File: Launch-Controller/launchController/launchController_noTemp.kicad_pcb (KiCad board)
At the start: 4 copper layers, 226 x 138.5 mm, 103 parts, among them J1 Conn_01x05_Pin, J10 Conn_01x05_Pin, J11 Raspberry_Pi_5, J13 26 pin Dsub, J14 DB25_Plug, J16 DB25_Plug, J17 DB25_Plug, J2 Conn_01x05_Pin, J3 Conn_01x05_Pin, J4 Conn_01x05_Pin, J5 Conn_01x05_Pin, J6 Conn_01x05_Pin, J7 Conn_01x05_Pin, J8 Conn_01x05_Pin, J9 Conn_01x05_Pin, Q1 NFET, Q10 NFET, Q2 NFET, Q3 NFET, Q4 NFET, Q5 NFET, Q6 NFET, Q7 NFET, Q8 NFET, Q9 NFET, U1 ADS1015IDGS, U2 ADS1015IDGS

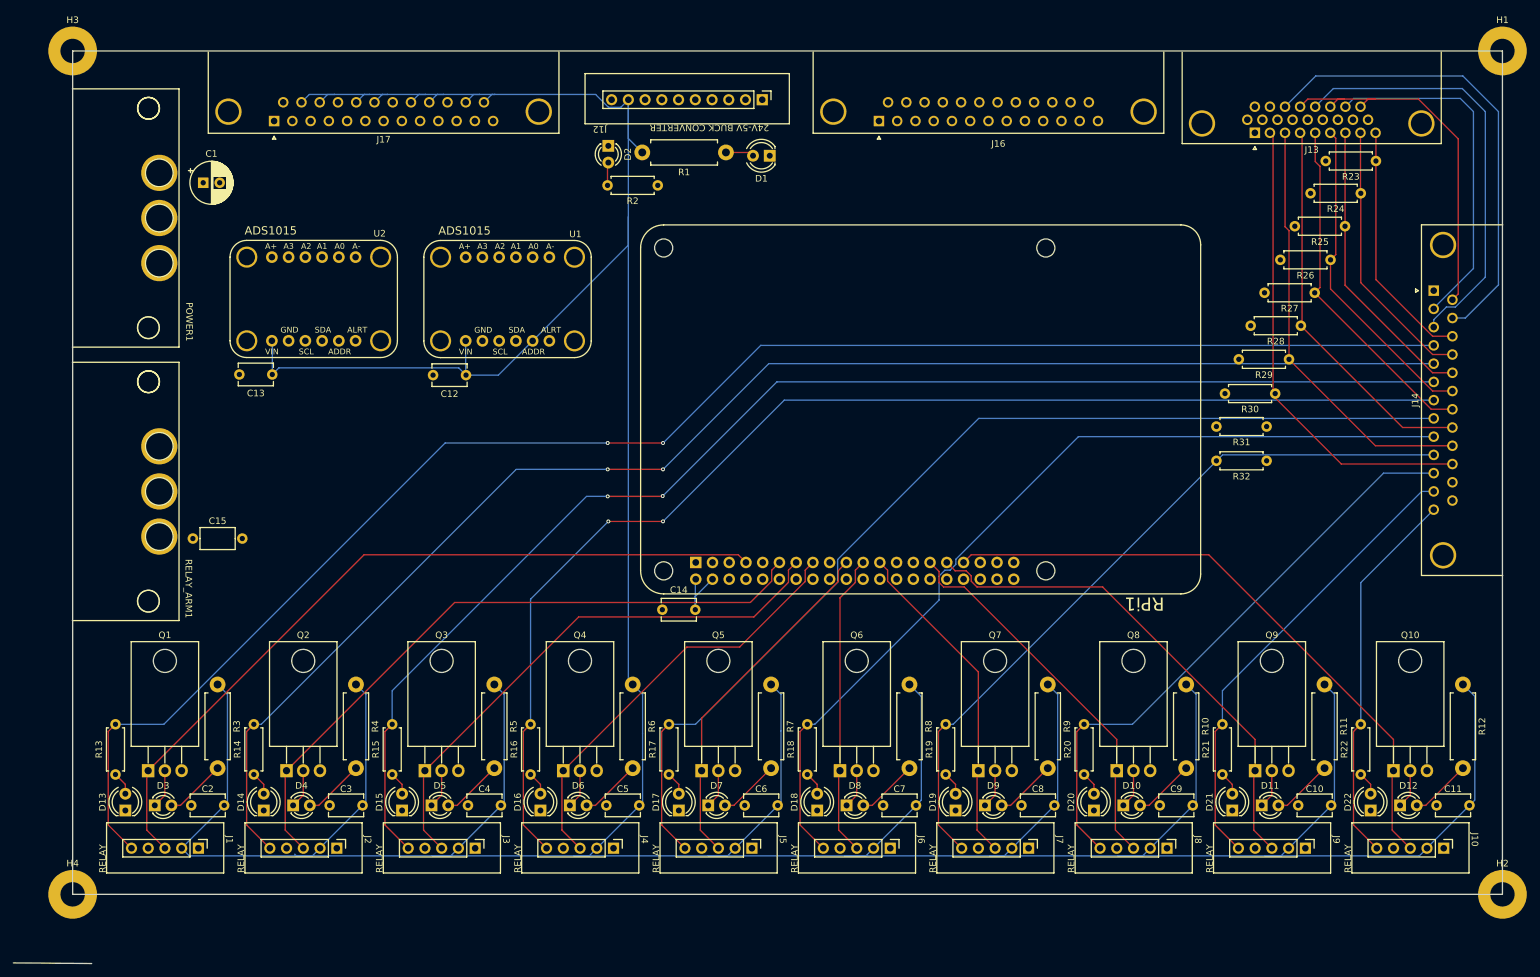
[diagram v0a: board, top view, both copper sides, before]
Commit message: dimensions
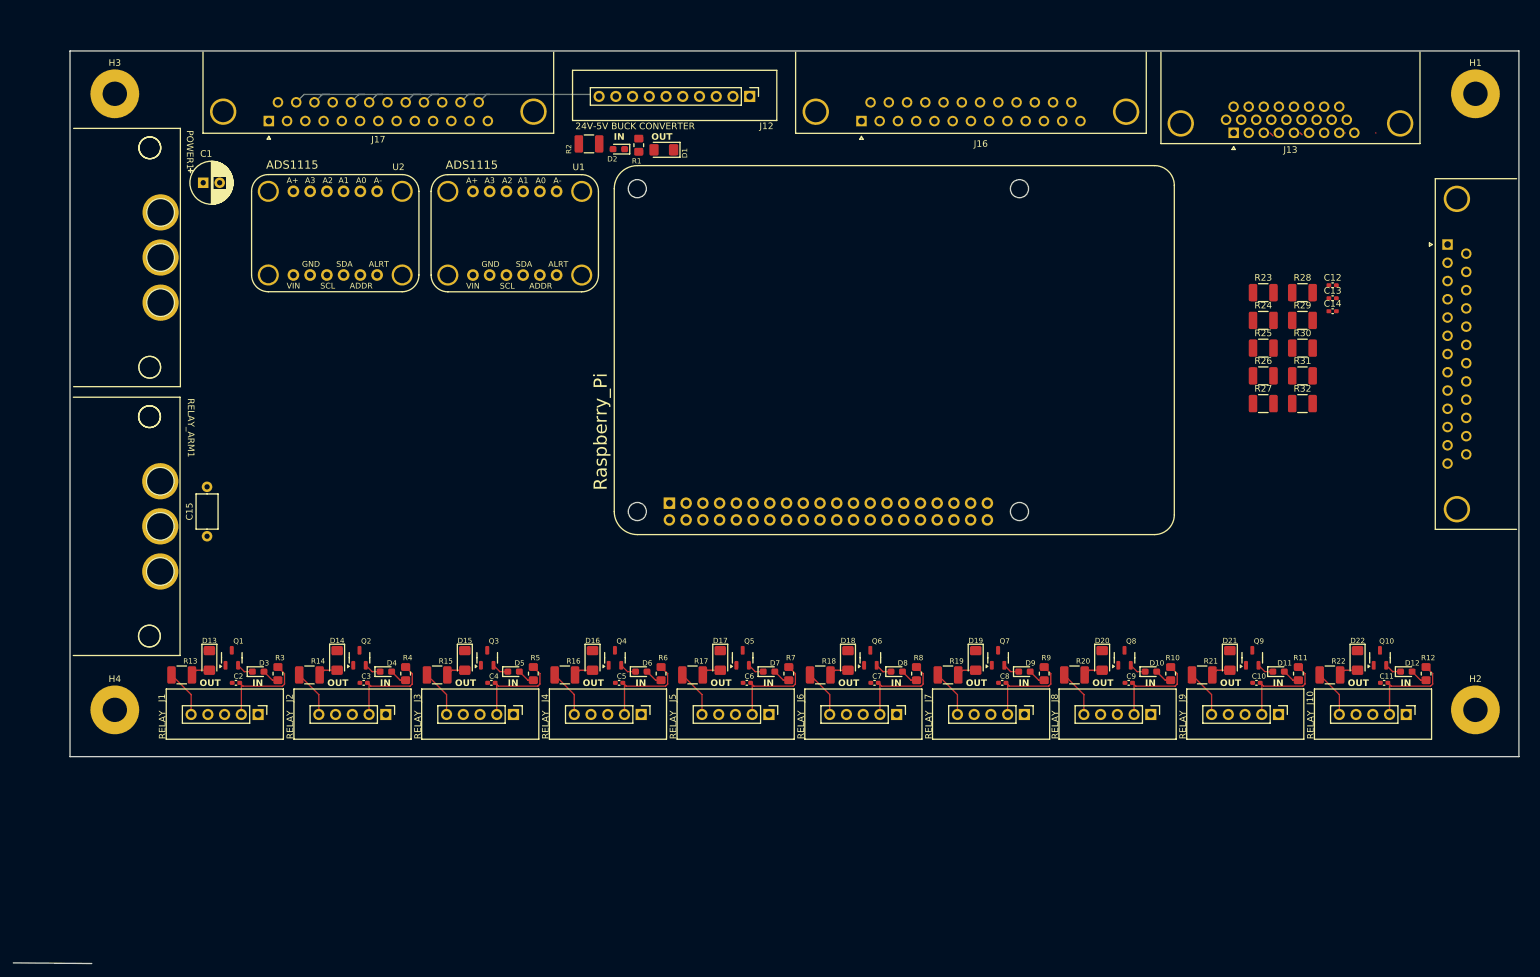
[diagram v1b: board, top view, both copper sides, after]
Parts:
- C10, C11, C12, C13, C14, C2, C3, C4, C5, C6, C7, C8, C9: footprint Capacitor_THT:C_Disc_D5.1mm_W3.2mm_P5.00mm -> Capacitor_SMD:C_0402_1005Metric_Pad0.74x0.62mm_HandSolder
- D1, D13, D14, D15, D16, D17, D18, D19, D20, D21, D22: footprint LED_THT:LED_D4.0mm -> LED_SMD:LED_1206_3216Metric_Pad1.42x1.75mm_HandSolder
- D10, D11, D12, D2, D3, D4, D5, D6, D7, D8, D9: footprint LED_THT:LED_D3.0mm -> LED_SMD:LED_0603_1608Metric_Pad1.05x0.95mm_HandSolder
- Q1, Q10, Q2, Q3, Q4, Q5, Q6, Q7, Q8, Q9: footprint Package_TO_SOT_THT:TO-220-3_Horizontal_TabDown -> Package_TO_SOT_SMD:SOT-23-3
- R1, R10, R11, R12, R3, R4, R5, R6, R7, R8, R9: footprint Resistor_THT:R_Axial_DIN0411_L9.9mm_D3.6mm_P12.70mm_Horizontal -> Resistor_SMD:R_0805_2012Metric_Pad1.20x1.40mm_HandSolder
- R13, R14, R15, R16, R17, R18, R19, R2, R20, R21, R22, R23, R24, R25, R26, R27, R28, R29, R30, R31, R32: footprint Resistor_THT:R_Axial_DIN0207_L6.3mm_D2.5mm_P7.62mm_Horizontal -> Resistor_SMD:R_1210_3225Metric_Pad1.30x2.65mm_HandSolder
- U1, U2: footprint SARP:ADS1015 -> launch_controller:ADS1115
- moved C13 161.3 mm to (381.7, 309.0), turned to 0 degrees
- moved C12 132.2 mm to (381.7, 307.1), turned to 0 degrees
- moved C14 106.8 mm to (381.7, 311.0), turned to 0 degrees
- moved H4 28.7 mm to (196.9, 371.5)
- moved H2 28.3 mm to (403.4, 371.5)
- moved R23 26.3 mm to (371.2, 308.2), turned to 0 degrees
- moved D13 26.1 mm to (211.3, 364.0), turned to -90 degrees
- moved D3 25.7 mm to (218.7, 365.7)
- moved D14 25.3 mm to (230.6, 364.0), turned to -90 degrees
- moved D4 24.7 mm to (238.0, 365.7)
- moved D15 24.7 mm to (250.0, 364.0), turned to -90 degrees
- moved R24 24.3 mm to (371.2, 312.4), turned to 0 degrees
- moved D16 24.1 mm to (269.4, 364.0), turned to -90 degrees
- moved D5 23.8 mm to (257.4, 365.7)
- moved D17 23.6 mm to (288.8, 364.0), turned to -90 degrees
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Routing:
- net /+5V: track 765.3 -> 213.6 mm
- net /RelayOut1: track 245.0 -> 7.23 mm, vias 2 -> 0
- net /RelayOut2: track 222.9 -> 7.23 mm, vias 2 -> 0
- net /RelayOut3: track 203.8 -> 7.23 mm, vias 2 -> 0
- net /RelayOut4: track 189.7 -> 7.23 mm, vias 2 -> 0
- net /RelayOut5: track 158.4 -> 7.23 mm
- net /RelayOut6: track 136.9 -> 7.23 mm
- net /GPIO 4: track 117.8 -> 0.00 mm
- net /RelayOut7: track 112.1 -> 7.23 mm
- net /GPIO 17: track 101.9 -> 0.00 mm
- net /GPIO 13: track 95.1 -> 0.00 mm
- net /GPIO 27: track 83.5 -> 0.00 mm
- net /RelayOut8: track 90.0 -> 7.23 mm
- net /GPIO 6: track 76.1 -> 0.00 mm
- net /PressureSwitch_in3: track 71.9 -> 0.00 mm
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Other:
- board size 226 x 138.5 mm -> 228.5 x 138.5 mm
- board text added: "IN"
- board text added: "OUT"
